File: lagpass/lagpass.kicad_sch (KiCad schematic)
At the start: 7 parts, among them U1 TL072

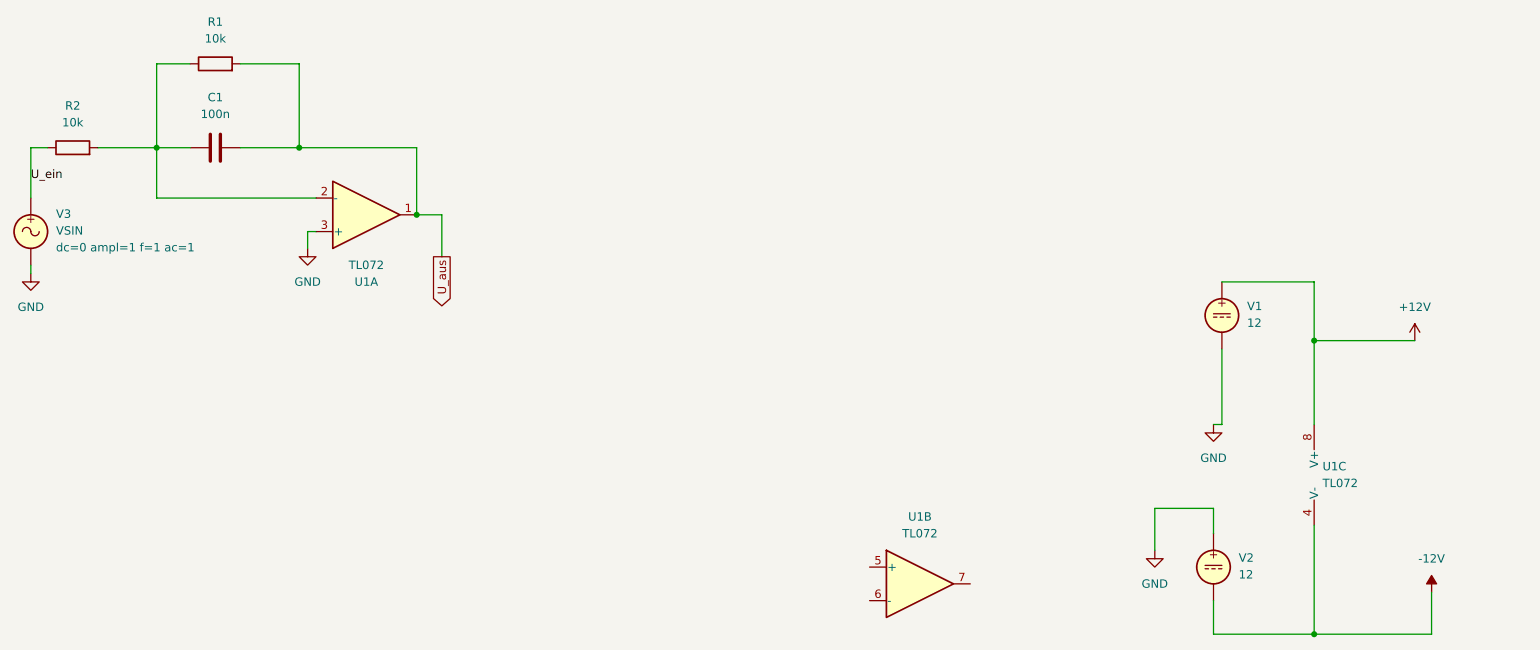
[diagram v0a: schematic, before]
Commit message: adding lagpass and allpass
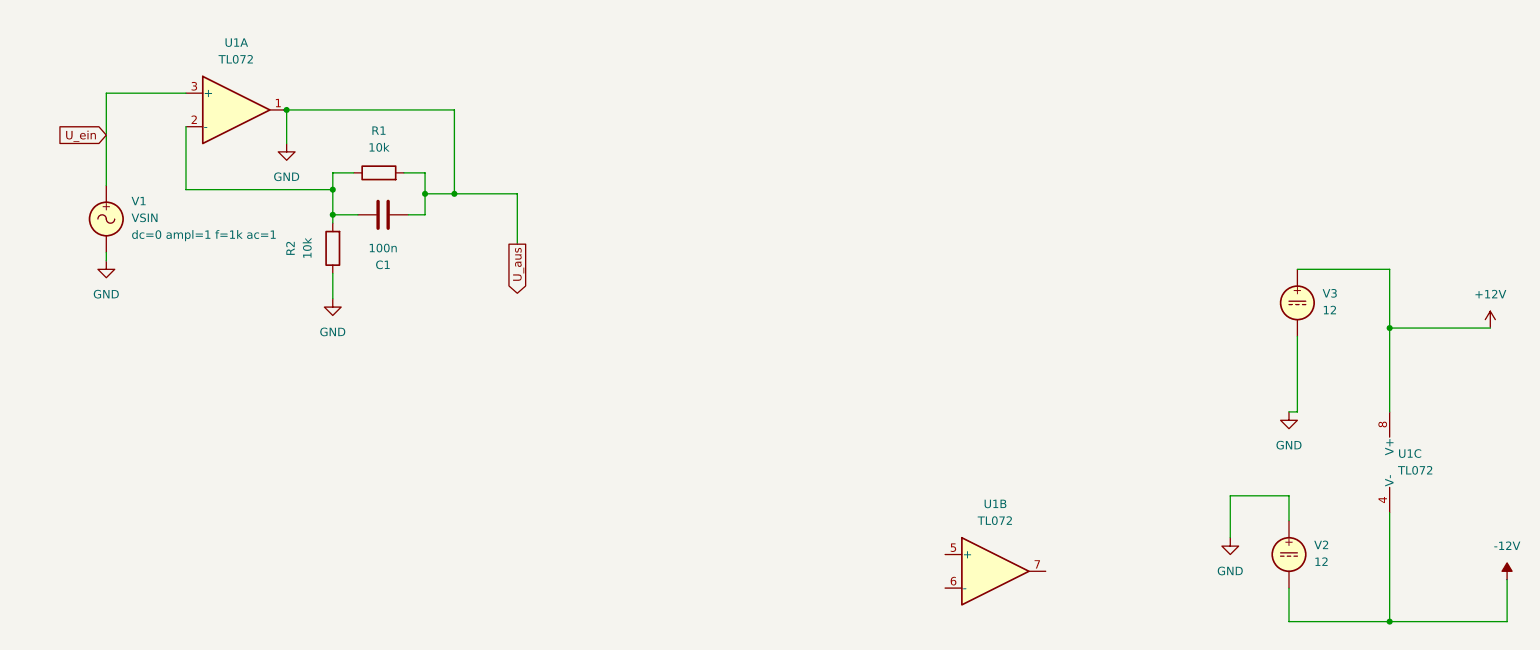
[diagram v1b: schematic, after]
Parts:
- removed V1: 12, symbol Simulation_SPICE:VDC
- removed V3: VSIN, symbol Simulation_SPICE:VSIN
- added V1: VSIN, symbol Simulation_SPICE:VSIN
- added V3: 12, symbol Simulation_SPICE:VDC
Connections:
- net U_aus is gone; now on net GND: C1.2, R1.2, U1.1
- net +12V: now also V3.1
- net GND: now also R2.1, V1.2, V3.2; no longer U1.3 (+)
- net U_ein: now also U1.3 (+), V1.1; no longer R2.1
